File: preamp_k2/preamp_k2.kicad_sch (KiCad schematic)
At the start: 23 parts, among them J1 AudioJack_Stereo, J2 AudioJack_Stereo, J3 9VDC, Q1 BC549, Q2 BC559, Q3 BC549

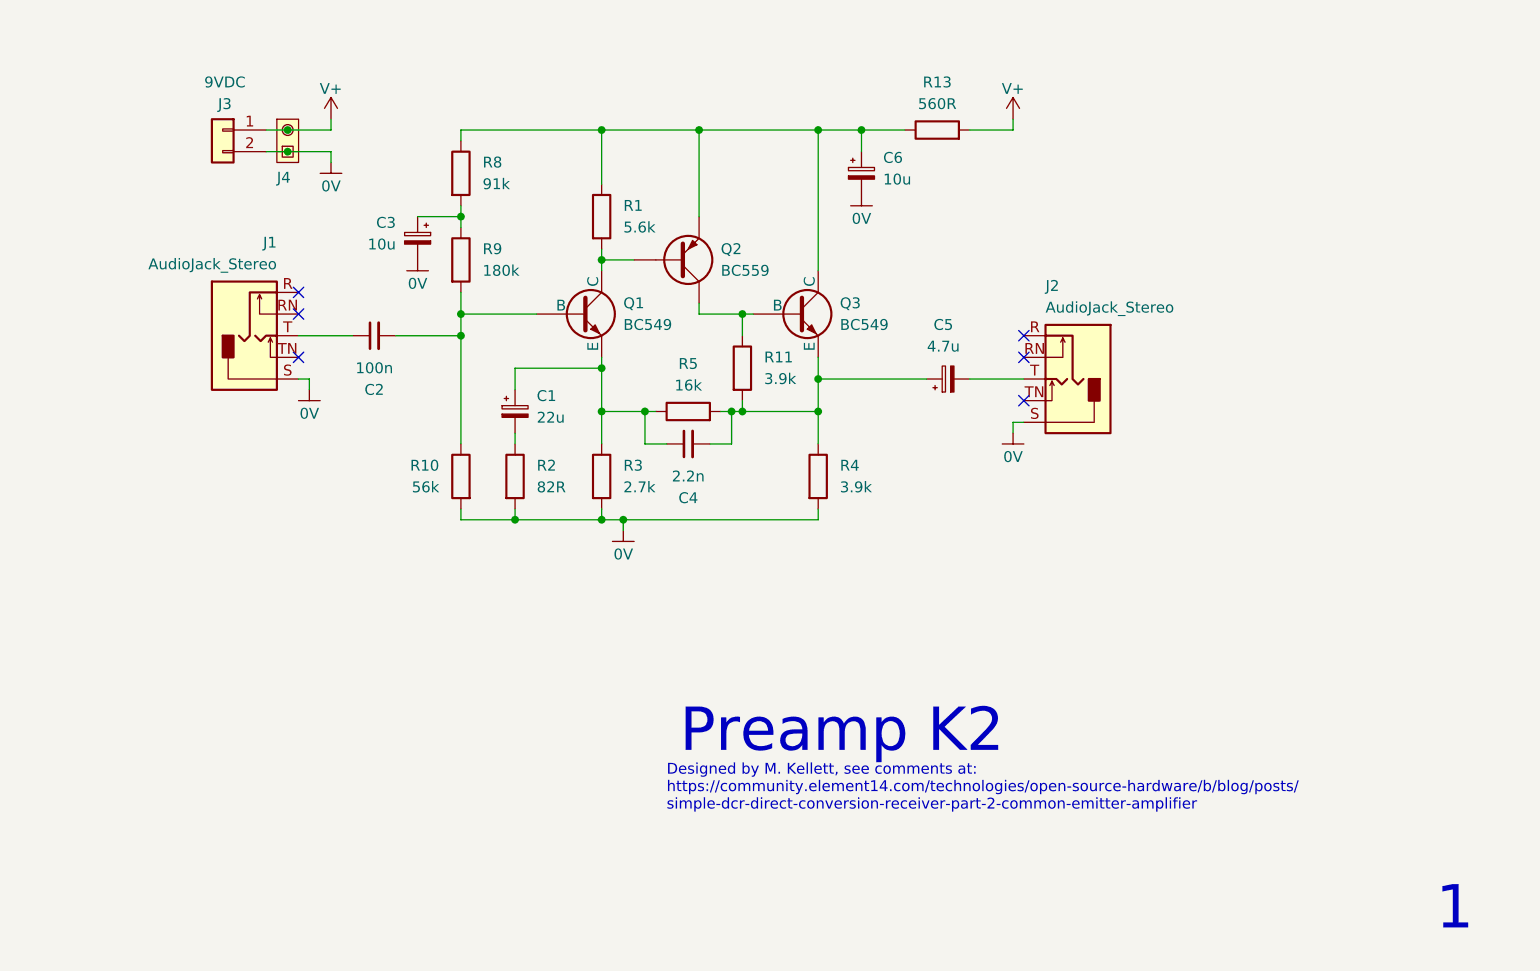
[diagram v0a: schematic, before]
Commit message: Add files via upload
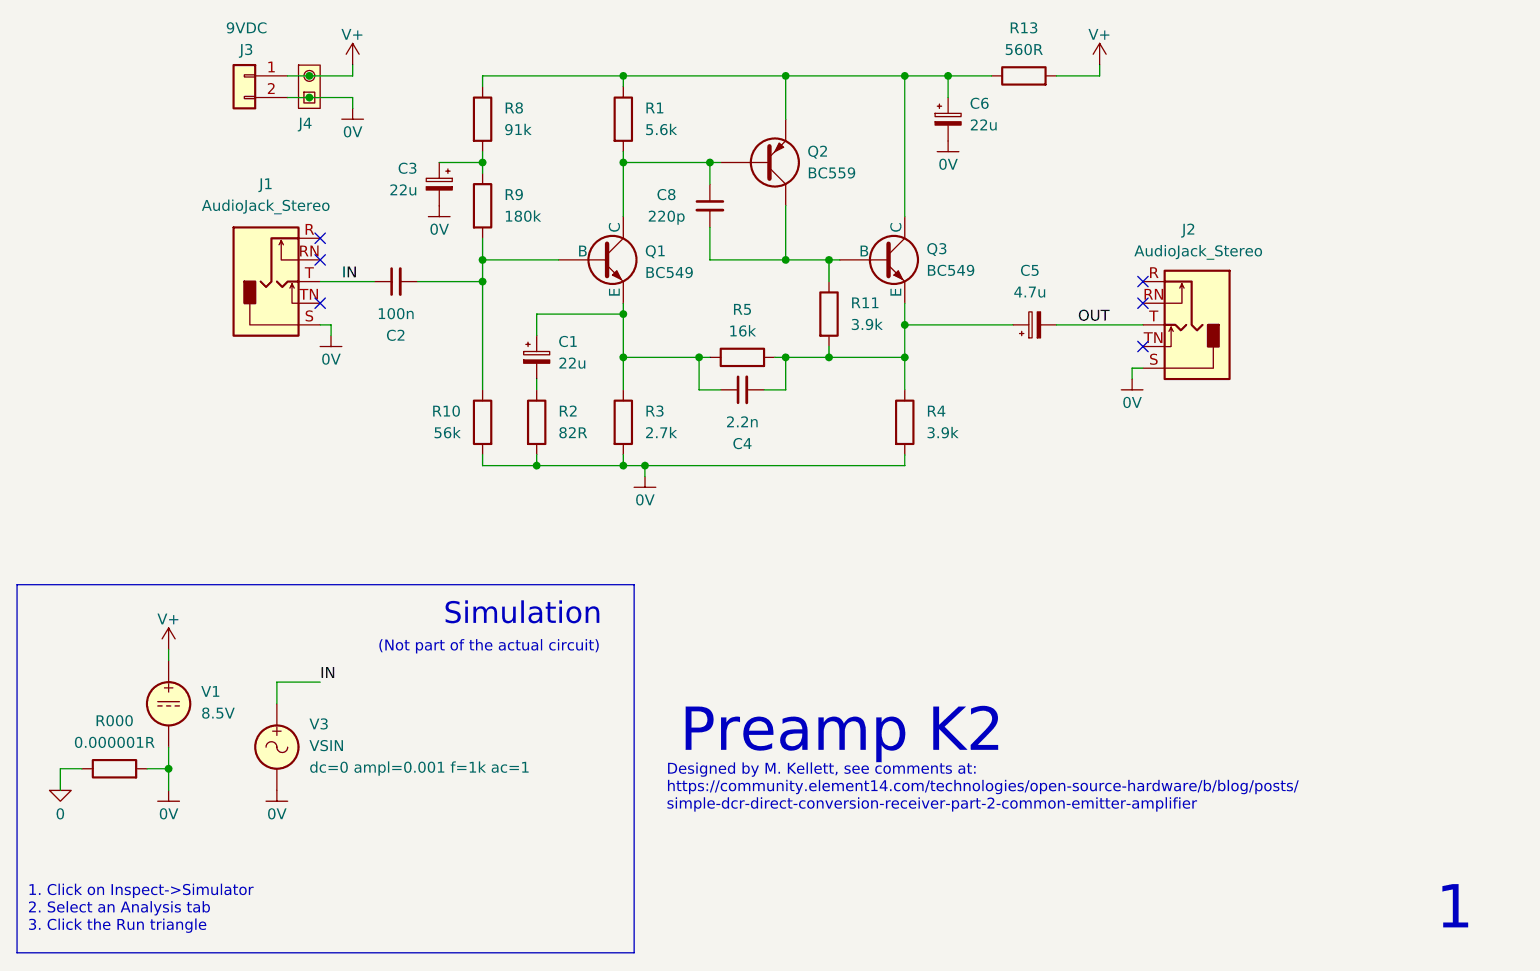
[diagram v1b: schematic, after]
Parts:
- added C8: 220p, User_Proto_Friendly:C_Disc_T3.0mm_P5.0, symbol USER_Proto_Friendly:C_Small
- added R000: 0.000001R, User_Proto_Friendly:R_Axial_L6.3mm_D2.5mm_P10.16mm_Horiz, symbol USER_Proto_Friendly:R
- added V1: 8.5V, symbol Simulation_SPICE:VDC
- added V3: VSIN, symbol Simulation_SPICE:VSIN
- C3, C6: value 10u -> 22u
- J4: footprint User_Proto_Friendly:PinHeader_1x02_P2.54mm_Vertical -> User_Global_Library:PinHeader_1x02_P2.54mm_Vertical
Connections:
- net 0V: now also R000.2, V1.2, V3.2
- net V+: now also V1.1
- net at Q2.1 (C), Q3.2 (B), R11.1: now also C8.2
- net at Q1.1 (C), Q2.2 (B), R1.2: now also C8.1
- net OUT: now reaches C5.2, J2.T
- net IN: now reaches C2.1, J1.T
- net IN: now also V3.1
- new net 0: R000.1
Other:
- note added: "(Not part of the actual circuit)"
- note added: "1. Click on Inspect->Simulator 2. Select an Analysis tab 3. Click the Run triangle"
- note added: "Simulation"
- moved on the sheet: C1, C2, C3, C4, C5, C6, J3, J4, Q1, Q2, Q3, R1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
